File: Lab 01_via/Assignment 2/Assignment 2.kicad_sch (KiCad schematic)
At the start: 6 parts, among them U1 AP2112K-3.3, U2 ESP32-S2-WROVER, U3 AL8860WT

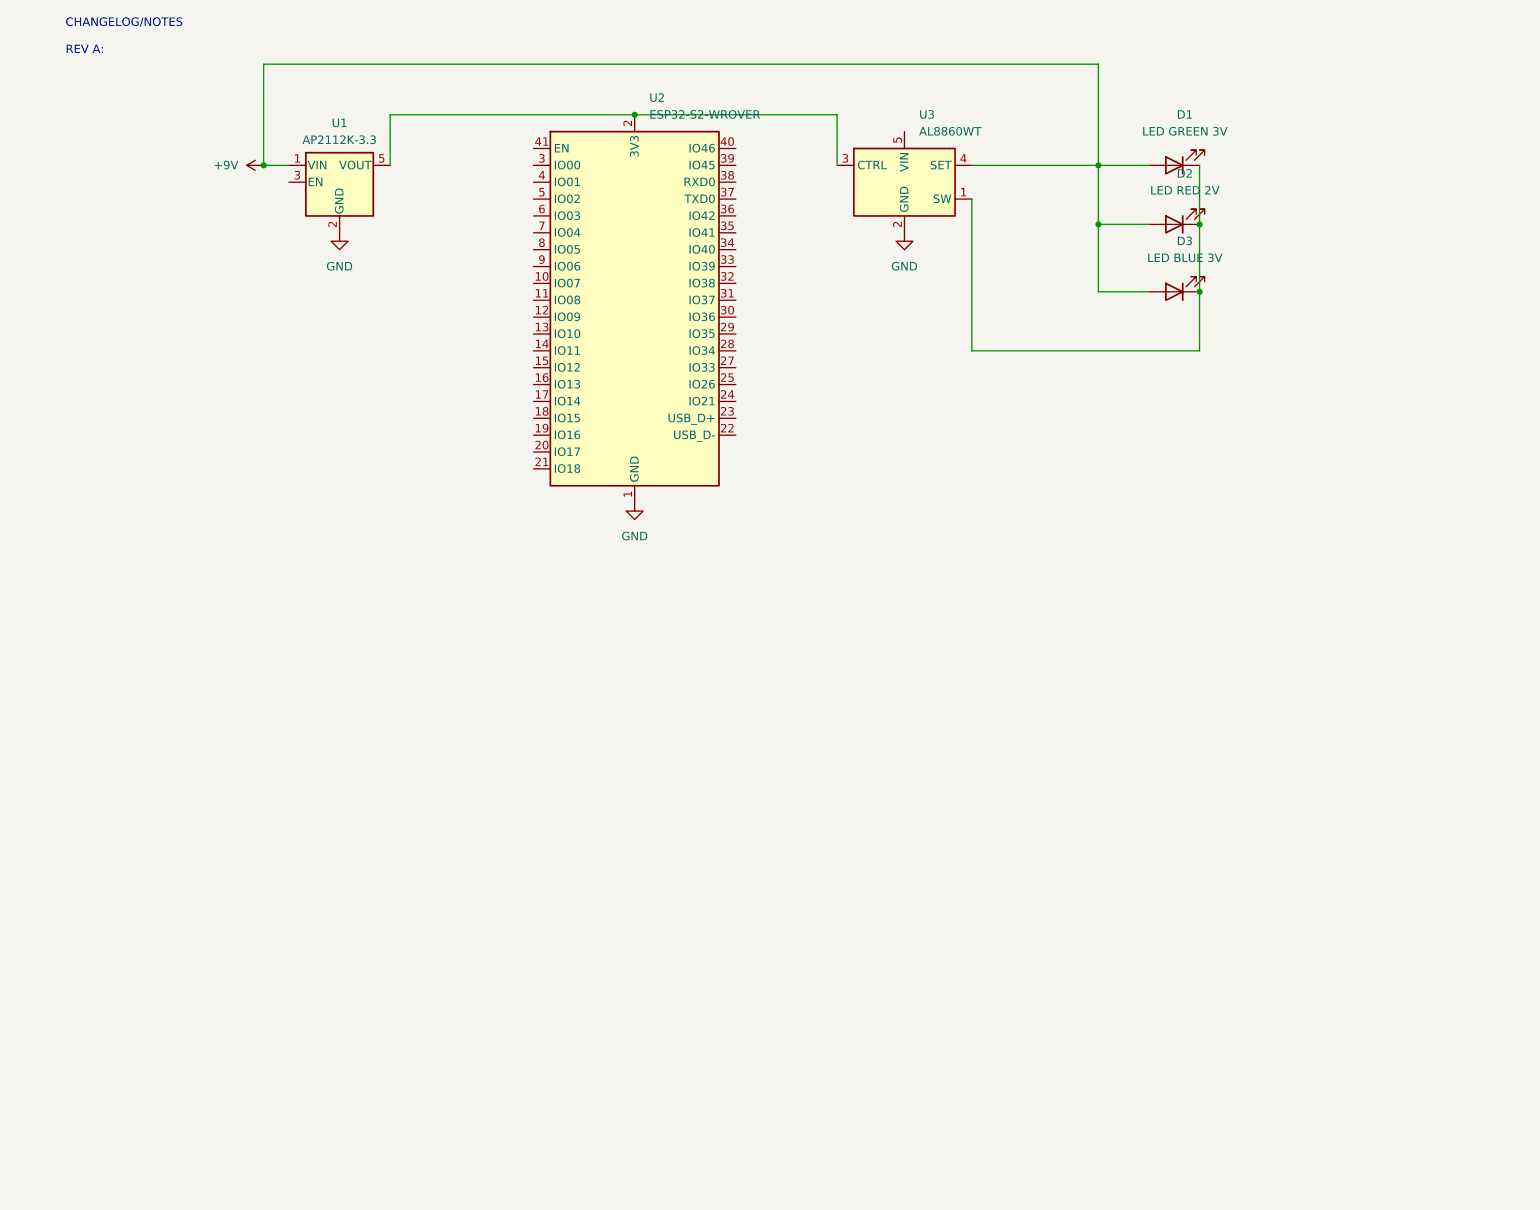
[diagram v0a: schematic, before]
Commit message: assignment 2 pls
this is gonna explode
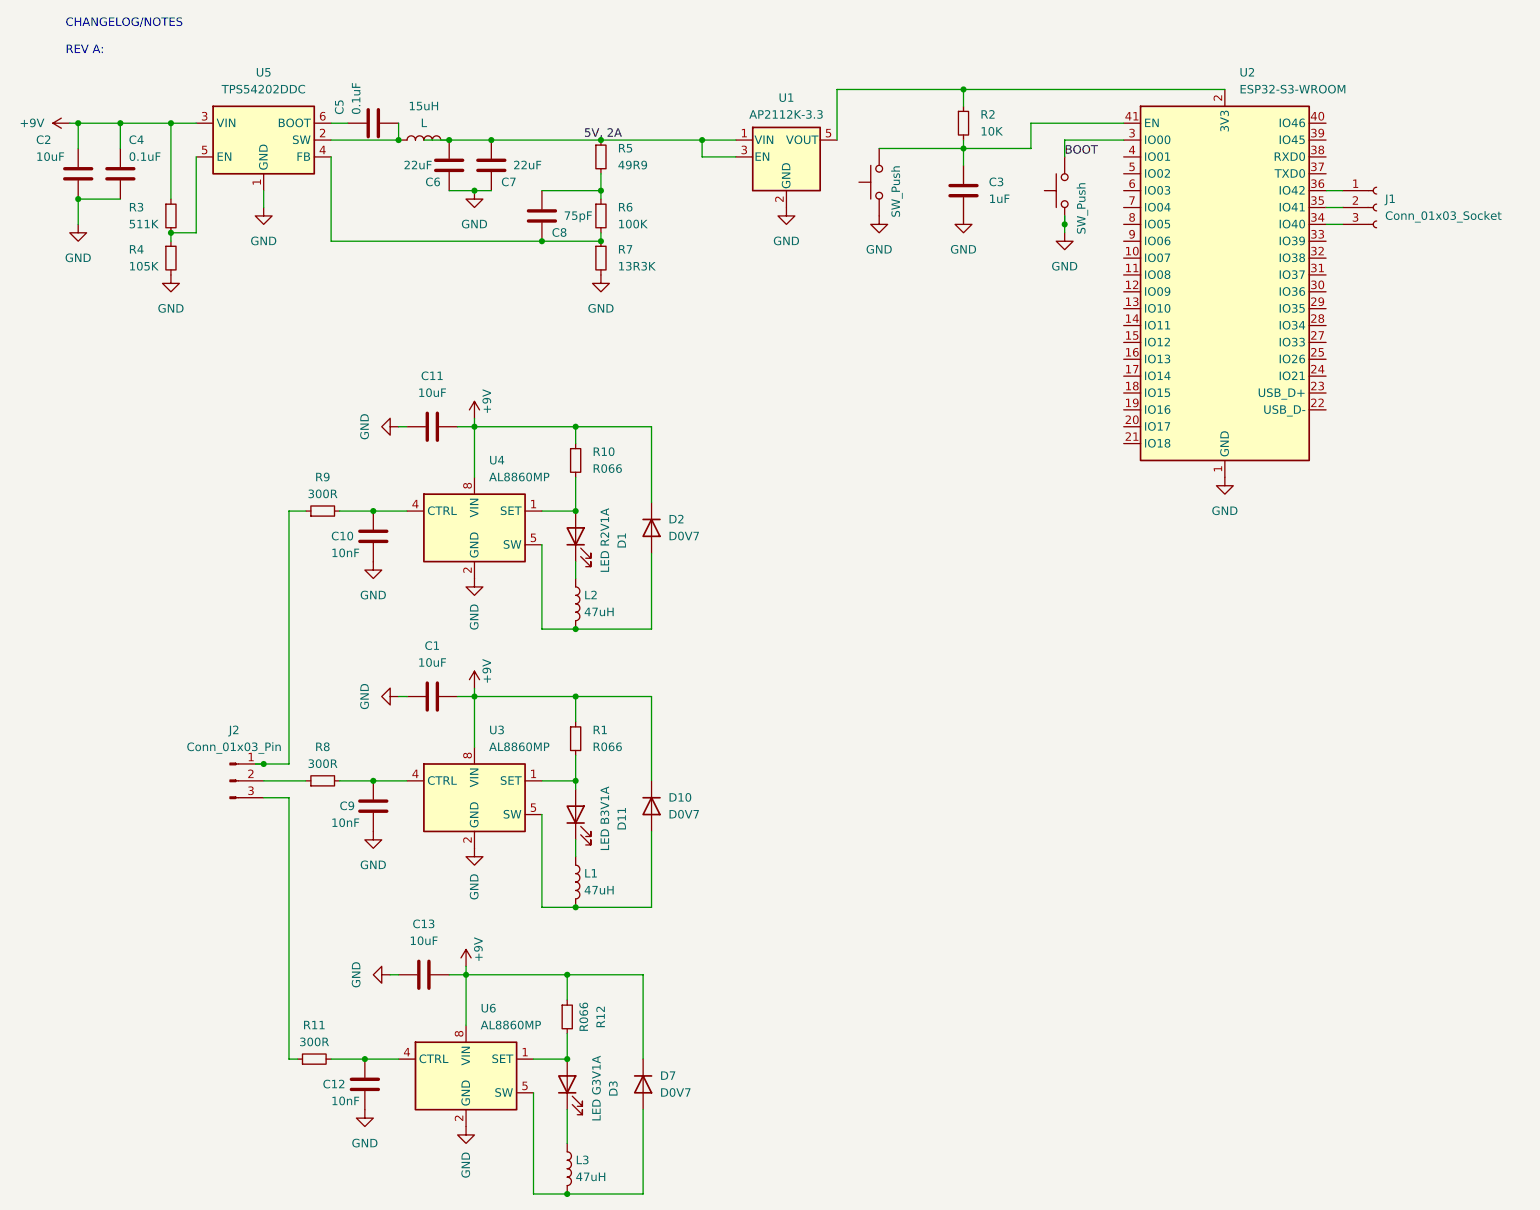
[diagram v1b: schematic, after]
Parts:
- removed D2: LED RED 2V, symbol Device:LED
- removed U3: AL8860WT, Package_TO_SOT_SMD:TSOT-23-5, symbol Driver_LED:AL8860WT
- added 15uH: L, symbol Device:L
- added C1, C11, C13, C2: 10uF, symbol Device:C
- added C10, C12, C9: 10nF, symbol Device:C
- added C3: 1uF, symbol Device:C
- added C4, C5: 0.1uF, symbol Device:C
- added C6, C7: 22uF, symbol Device:C
- added C8: 75pF, symbol Device:C
- added D10, D2, D7: D0V7, symbol Device:D
- added D11: LED B3V1A, symbol Device:LED
- added J1: Conn_01x03_Socket, symbol Connector:Conn_01x03_Socket
- added J2: Conn_01x03_Pin, symbol Connector:Conn_01x03_Pin
- added L1, L2, L3: 47uH, symbol Device:L
- added R1, R10, R12: R066, symbol Device:R_Small
- added R11, R8, R9: 300R, symbol Device:R_Small
- added R2: 10K, symbol Device:R_Small
- added R3: 511K, symbol Device:R_Small
- added R4: 105K, symbol Device:R_Small
- added R5: 49R9, symbol Device:R_Small
- added R6: 100K, symbol Device:R_Small
- added R7: 13R3K, symbol Device:R_Small
- added SW1, SW2: SW_Push, symbol Switch:SW_Push
- added U3, U4, U6: AL8860MP, Package_SO:MSOP-8-1EP_3x3mm_P0.65mm_EP1.5x1.8mm, symbol Driver_LED:AL8860MP
- added U5: TPS54202DDC, Package_TO_SOT_SMD:SOT-23-6, symbol Regulator_Switching:TPS54202DDC
- D1: value LED GREEN 3V -> LED R2V1A
- D3: value LED BLUE 3V -> LED G3V1A
- U2: value ESP32-S2-WROVER -> ESP32-S3-WROOM; footprint RF_Module:ESP32-S2-WROVER -> Library:XCVR_ESP32-S3-WROOM-1-N4
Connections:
- net +9V: now also C1.1, C11.1, C13.1, C2.2, C4.2, D10.1 (K), D2.1 (K), D7.1 (K), R1.1, R10.1, R12.1, R3.1, U3.8 (VIN), U4.8 (VIN), U5.3 (VIN), U6.8 (VIN); no longer D1.2 (A), D3.2 (A), U1.1 (VIN)
- net GND: now also C1.2, C10.2, C11.2, C12.2, C13.2, C2.1, C3.1, C4.1, C6.2, C7.2, C9.2, R4.2, R7.2, SW1.1, SW2.1, U3.2 (GND), U3.3 (GND), U3.9 (GND), U4.2 (GND), U4.3 (GND), U4.9 (GND), U5.1 (GND), U6.2 (GND), U6.3 (GND), U6.9 (GND)
- net at D1.1 (K): now also L2.1; no longer D3.1 (K)
- net at U1.5 (VOUT), U2.2 (3V3): now also R2.1
- net BOOT: now reaches U2.3 (IO00)
- net BOOT: now also SW2.2
- net at U2.34 (IO40): now also J1.3 (Pin_3)
- net at U2.35 (IO41): now also J1.2 (Pin_2)
- net at U2.36 (IO42): now also J1.1 (Pin_1)
- net at U2.41 (EN): now also C3.2, R2.2, SW1.2
- net 5V, 2A: now reaches U1.3 (EN)
- net 5V, 2A: now also U1.1 (VIN), 15uH.2, C6.1, C7.1, R5.1
- new net: R3.2, R4.1, U5.5 (EN)
- new net: J2.2 (Pin_2), R8.1
- new net: C9.1, R8.2, U3.4 (CTRL)
- new net: 15uH.1, C5.1, U5.2 (SW)
- new net: C5.2, U5.6 (BOOT)
- new net: D2.2 (A), L2.2, U4.5 (SW), U4.6 (SW)
- new net: D7.2 (A), L3.2, U6.5 (SW), U6.6 (SW)
- new net: C10.1, R9.2, U4.4 (CTRL)
- new net: D11.1 (K), L1.1
- new net: D11.2 (A), R1.2, U3.1 (SET)
- new net: D1.2 (A), R10.2, U4.1 (SET)
- new net: C8.2, R6.2, R7.1, U5.4 (FB)
- new net: D10.2 (A), L1.2, U3.5 (SW), U3.6 (SW)
- new net: D3.1 (K), L3.1
- new net: D3.2 (A), R12.2, U6.1 (SET)
- new net: C8.1, R5.2, R6.1
- new net: C12.1, R11.2, U6.4 (CTRL)
- new net: J2.1 (Pin_1), R9.1
- new net: J2.3 (Pin_3), R11.1
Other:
- moved on the sheet: U1
